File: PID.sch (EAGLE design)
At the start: 32 parts, among them IC1 MC78M05ABT, IC2 MC79M05BT, X3 1-227161-0, X4 1-227161-0

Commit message: 2019/3/31更新
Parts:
- added C11, C12, C14, C15, C16, C17, C18, C19, C20, C28, C29, C30, C31, C32, C33, C34, C35, C36, C37, C38, C39, C40, C41, C42, C43, C44, C45, C46, C47, C48, C49, C50: (no value), rcl:C-EUC0603
- added INPUT1, INPUT2: 1-227161-0, con-coax:1-227161-0
- added R10, R11, R12, R13, R15, R16, R17, R18, R19, R20, R21, R22, R7, R8, R9: (no value), rcl:R-EU_R0603
- added R14: 51R, rcl:R-EU_R0603
- added SW3, SW4: (no value), special:SW_DIP-10
- added U$2, U$3: OPA656, Mylib:OPA656
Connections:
- new net N$16: C11.1, C12.2, R5.1, R7.2, R8.2, R9.1, U$1.VOUT
- new net N$17: R7.1
- new net N$19: INPUT.1, R1.2, U$1.P
- new net N$20: C50.1, R10.2, R11.2, R12.1, R13.1, R22.1, U$2.N
- new net N$21: C12.1, R10.1, R9.2
- new net N$22: U$2.VOUT
- new net N$23: R11.1, R15.1, R16.2
- new net N$24: C14.1, C15.1, C16.1, C17.1, C18.1, C19.1, C20.1, C28.1, C29.1, C50.2, R22.2
- new net N$25: C30.1, C31.1, C32.1, C33.1, C34.1, C35.1, C36.1, C37.1, C38.1
- new net N$26: C39.1, C40.1, C41.1, C42.1, C43.1, C44.1, C45.1, C46.1, C47.1
- new net N$27: U$2.VDD
- new net N$28: U$2.VSS
- new net N$29: INPUT1.1, R16.1, R17.2
- new net N$30: INPUT1.2, R15.2
- new net N$31: R21.2
- new net N$32: U$3.VSS
- new net N$33: C48.2, R20.2, R21.1, SW4.10, SW4.2, SW4.3, SW4.4, SW4.5, SW4.6, SW4.7, SW4.8, SW4.9, U$3.VOUT
- new net N$34: U$3.VDD
- new net N$35: C49.2, R18.2, R19.1
- new net N$36: U$3.P
- new net N$37: C48.1, R19.2, R20.1, U$3.N
- new net N$39: C30.2, C31.2, C32.2, C33.2, C34.2, C35.2, C36.2, C37.2, C38.2, R14.2, R17.1
- new net N$40: R13.2
- new net N$41: INPUT2.1
- net 0: now also C49.1, INPUT.2, INPUT2.2, R18.1
- net N$13: now also C11.2, R3.2, R8.1, U$1.N

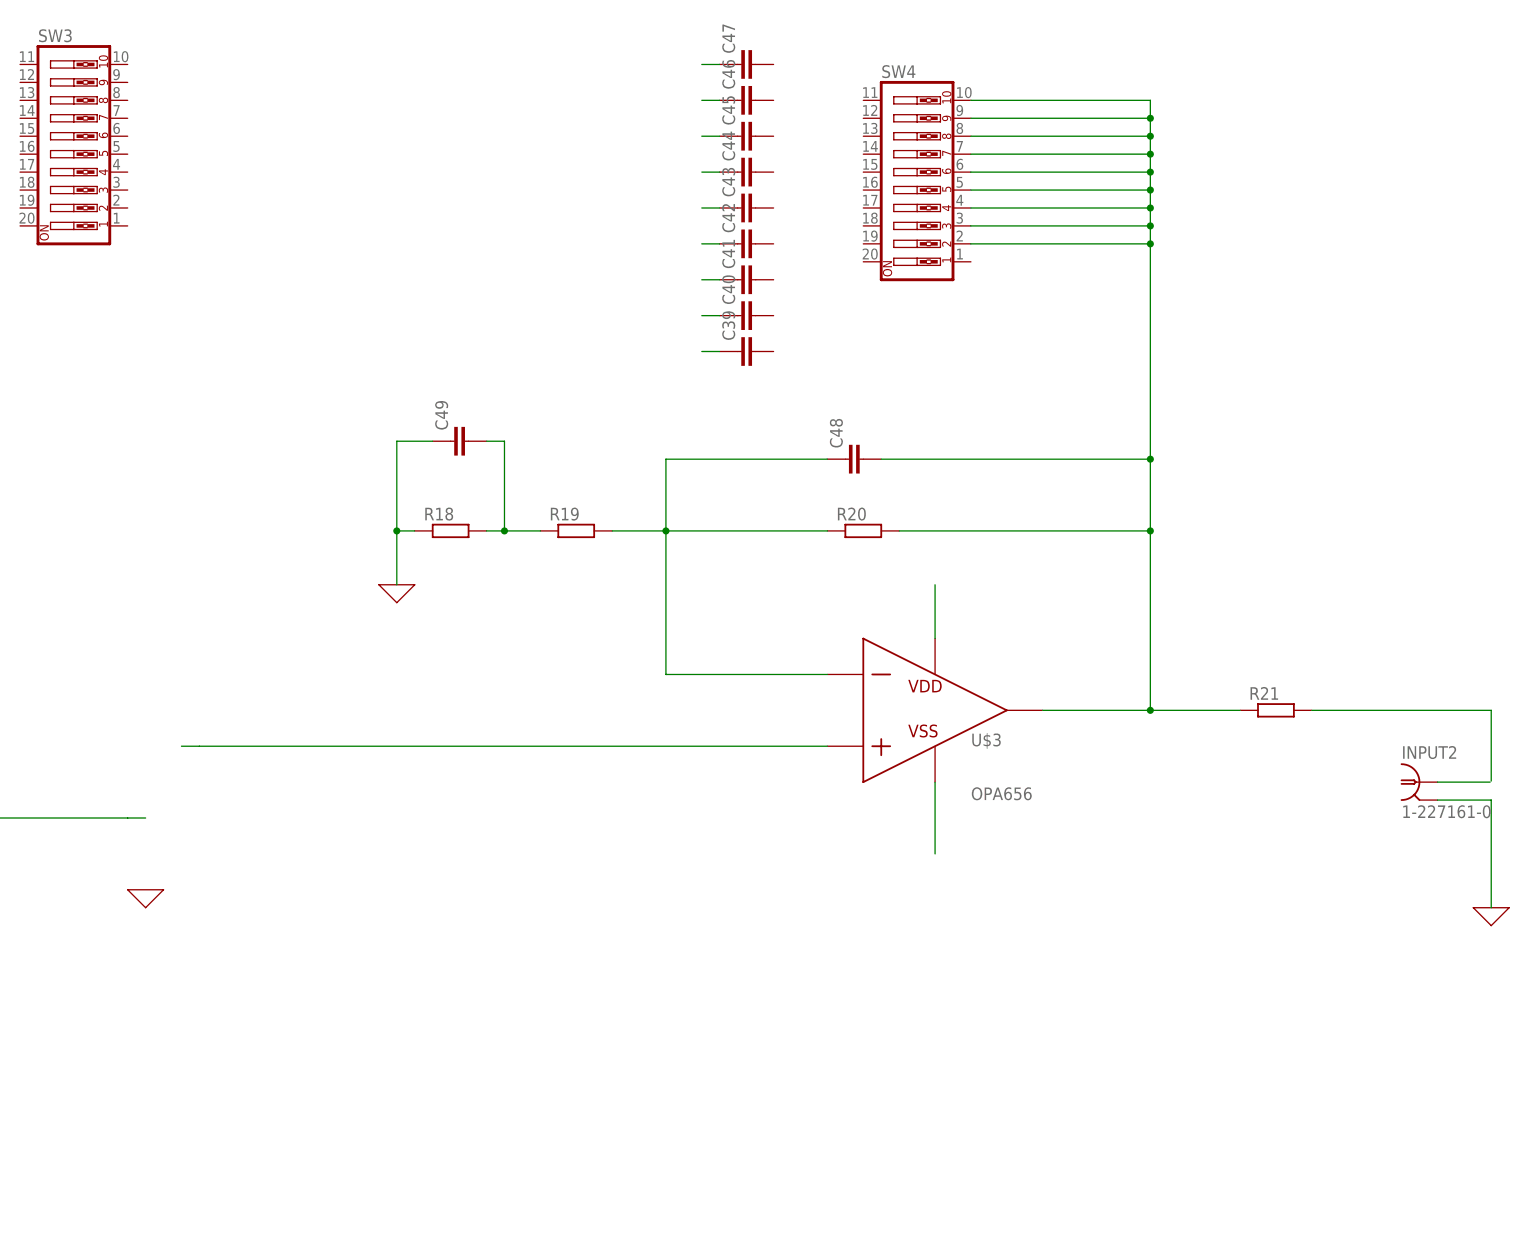
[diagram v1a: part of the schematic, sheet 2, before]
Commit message: 2019/04/15 Update
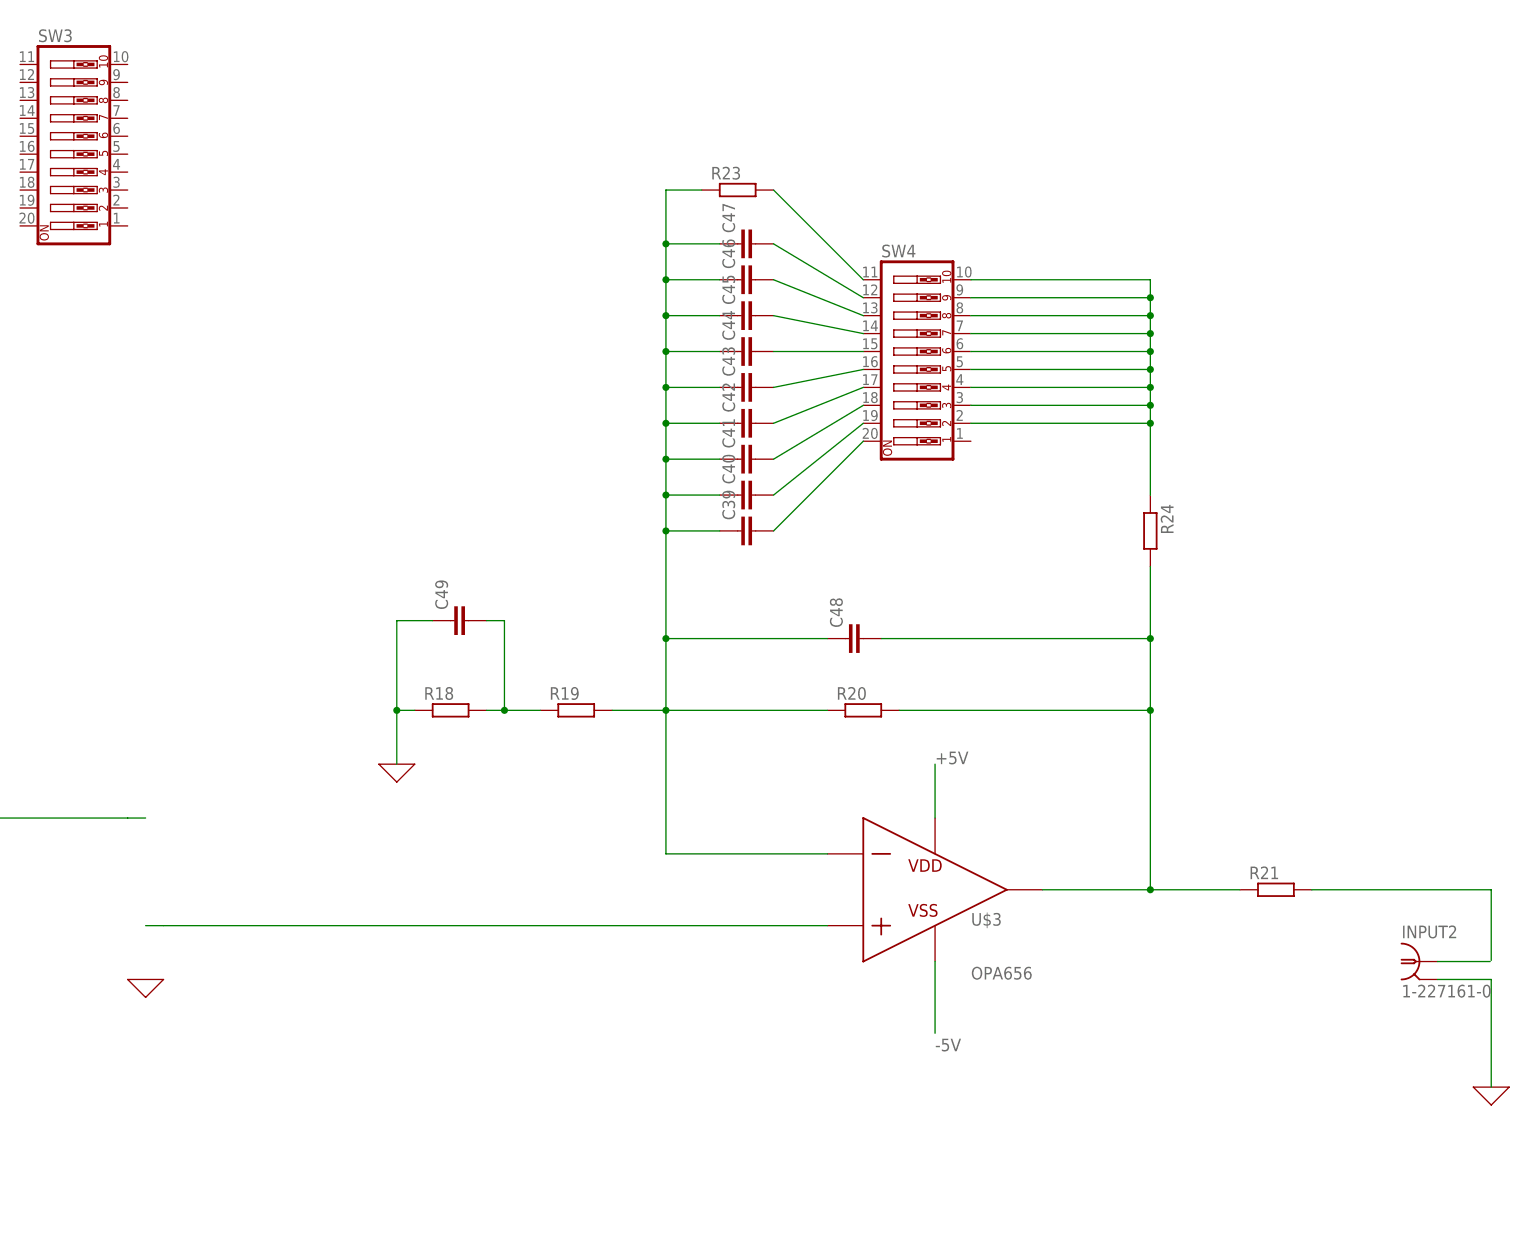
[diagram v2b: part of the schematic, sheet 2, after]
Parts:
- added R23, R24: (no value), rcl:R-EU_R0603
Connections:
- removed net N$32: U$3.VSS
- removed net N$34: U$3.VDD
- new net N$38: C40.2, SW4.19
- new net N$42: C41.2, SW4.18
- new net N$43: C42.2, SW4.17
- new net N$44: C43.2, SW4.16
- new net N$45: C44.2, SW4.15
- new net N$46: C45.2, SW4.14
- new net N$47: C46.2, SW4.13
- new net N$48: C47.2, SW4.12
- new net N$50: R23.2, SW4.11
- new net N$51: C48.2, R20.2, R21.1, R24.2, U$3.VOUT
- net +5V: now also U$3.VDD
- net -5V: now also U$3.VSS
- net N$26: now also C39.2, SW4.20; no longer C39.1, C40.1, C41.1, C42.1, C43.1, C44.1, C45.1, C46.1, C47.1
- net N$33: now also R24.1; no longer C48.2, R20.2, R21.1, U$3.VOUT
- net N$37: now also C39.1, C40.1, C41.1, C42.1, C43.1, C44.1, C45.1, C46.1, C47.1, R23.1
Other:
- moved on the sheet: C39, C40, C41, C42, C43, C44, C45, C46, C47, C48, C49, INPUT2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
